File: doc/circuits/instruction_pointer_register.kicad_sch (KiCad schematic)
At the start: 8 parts, among them U1 74LS193, U10 74LS193, U2 74LS193, U3 74LS245, U4 74LS04, U5 74LS04, U8 74LS193, U9 74LS245

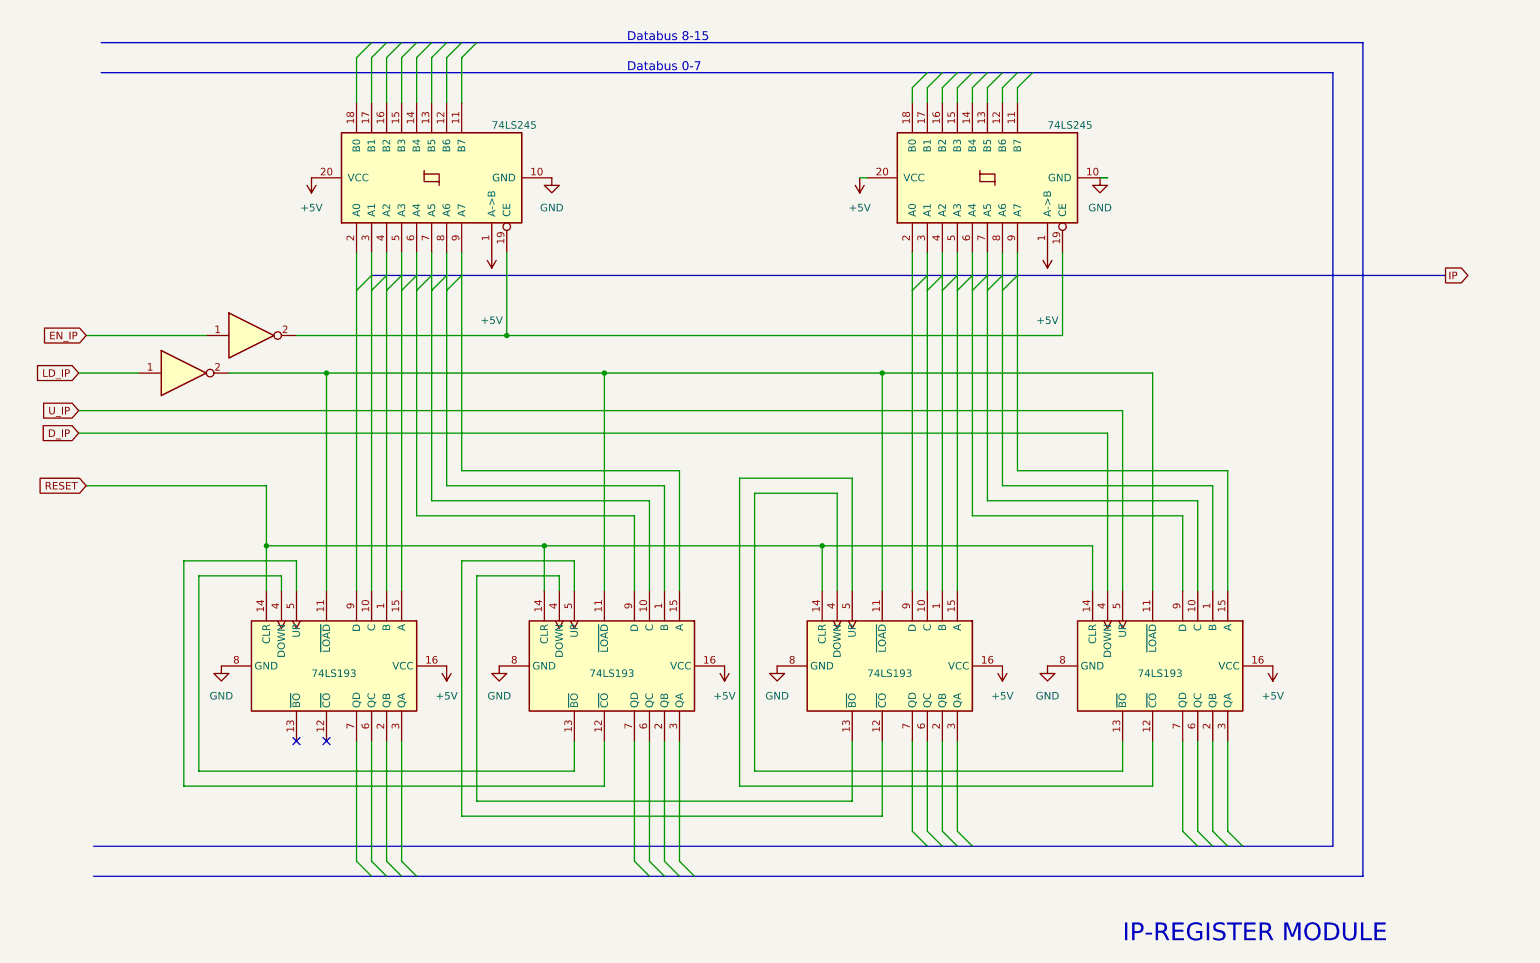
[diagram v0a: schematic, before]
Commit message: Updated schematics
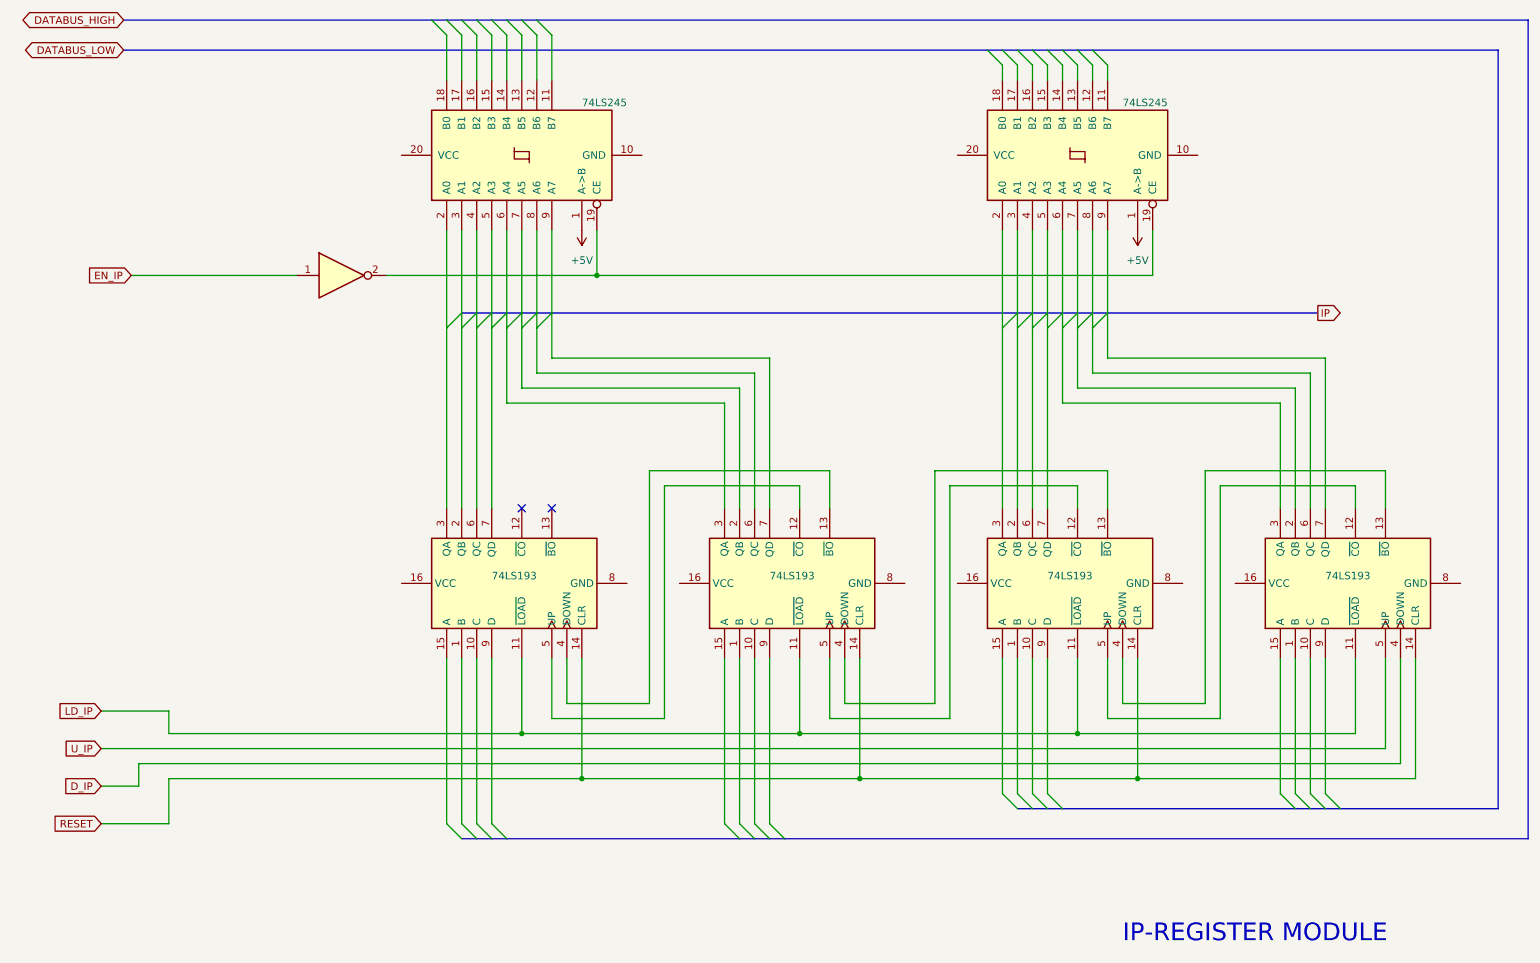
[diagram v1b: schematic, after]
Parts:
- removed U1, U10, U2, U8: 74LS193, symbol 74xx:74LS193
- removed U3, U9: 74LS245, symbol 74xx:74LS245
- removed U4, U5: 74LS04, symbol 74xx:74LS04
- added U11, U14: 74LS245, symbol 74xx:74LS245
- added U12, U13, U15, U7: 74LS193, symbol 74xx:74LS193
- added U6: 74LS04, symbol 74xx:74LS04
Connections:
- net +5V: now also U11.1 (A->B), U14.1 (A->B)
- net D_IP: now also U15.4 (DOWN)
- net EN_IP: now also U6.1
- net LD_IP: now also U12.11 (~{LOAD}), U13.11 (~{LOAD}), U15.11 (~{LOAD}), U7.11 (~{LOAD})
- net RESET: now also U12.14 (CLR), U13.14 (CLR), U15.14 (CLR), U7.14 (CLR)
- net U_IP: now also U15.5 (UP)
- new net: U11.3 (A1), U7.2 (QB)
- new net: U11.2 (A0), U7.3 (QA)
- new net: U12.13 (~{BO}), U7.4 (DOWN)
- new net: U12.12 (~{CO}), U7.5 (UP)
- new net: U11.4 (A2), U7.6 (QC)
- new net: U11.5 (A3), U7.7 (QD)
- new net: U11.7 (A5), U12.2 (QB)
- new net: U11.6 (A4), U12.3 (QA)
- new net: U12.4 (DOWN), U13.13 (~{BO})
- new net: U12.5 (UP), U13.12 (~{CO})
- new net: U11.8 (A6), U12.6 (QC)
- new net: U11.9 (A7), U12.7 (QD)
- new net: U11.19 (CE), U14.19 (CE), U6.2
- new net: U13.5 (UP), U15.12 (~{CO})
- new net: U13.4 (DOWN), U15.13 (~{BO})
- new net: U14.7 (A5), U15.2 (QB)
- new net: U14.6 (A4), U15.3 (QA)
- new net: U14.8 (A6), U15.6 (QC)
- new net: U14.9 (A7), U15.7 (QD)
- new net: U13.2 (QB), U14.3 (A1)
- new net: U13.3 (QA), U14.2 (A0)
- new net: U13.6 (QC), U14.4 (A2)
- new net: U13.7 (QD), U14.5 (A3)
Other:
- note removed: "Databus 0-7"
- note removed: "Databus 8-15"
